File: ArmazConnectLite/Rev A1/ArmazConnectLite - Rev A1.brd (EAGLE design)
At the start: 56 x 24 mm, 17 parts, among them J1 22-05-7028-02, X1 MSTBA3, X8 87832-26

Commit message: Place copyright and board name
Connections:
- new net +24V: X1.1
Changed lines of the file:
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@@
 <contactref element="X8" pad="17"/>
+</signal>
+<signal name="+24V">
+<contactref element="X1" pad="1"/>
 </signal>
 </signals>

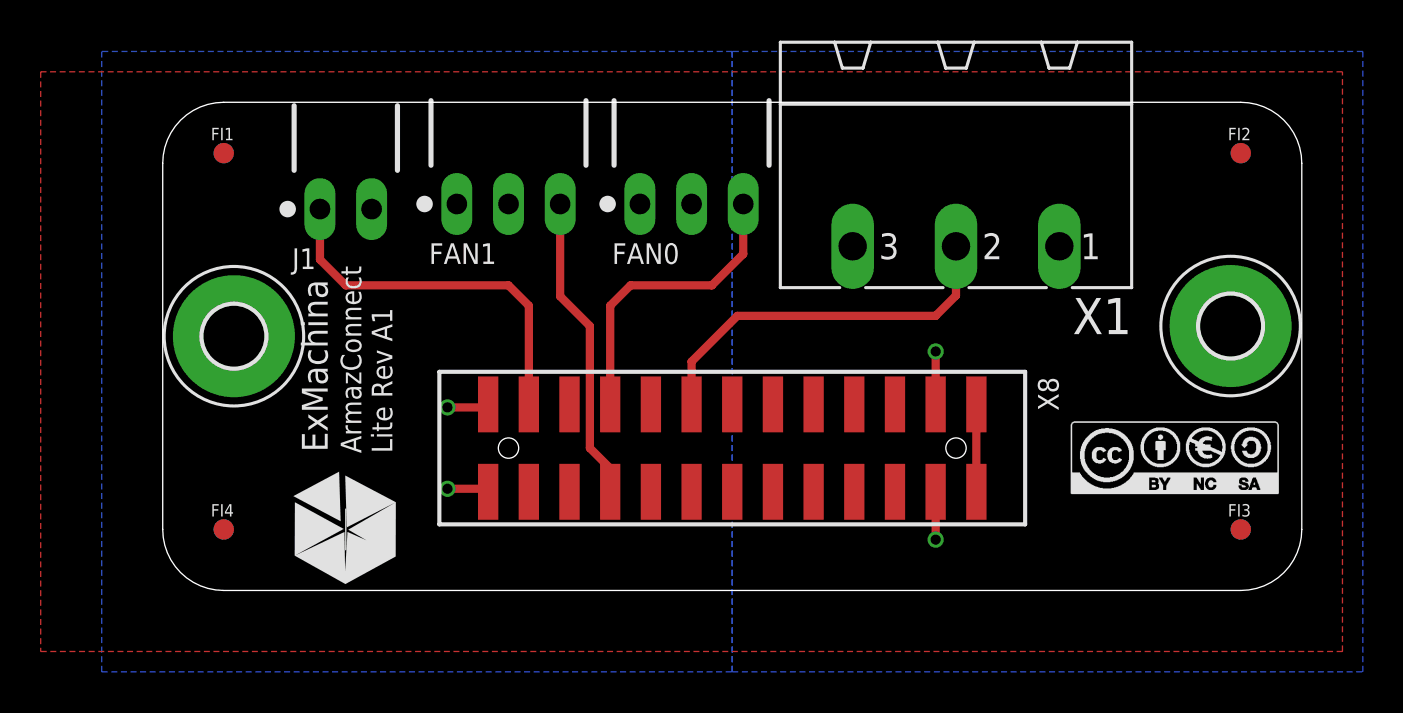
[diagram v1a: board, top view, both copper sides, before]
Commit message: generate gerber and MDP files
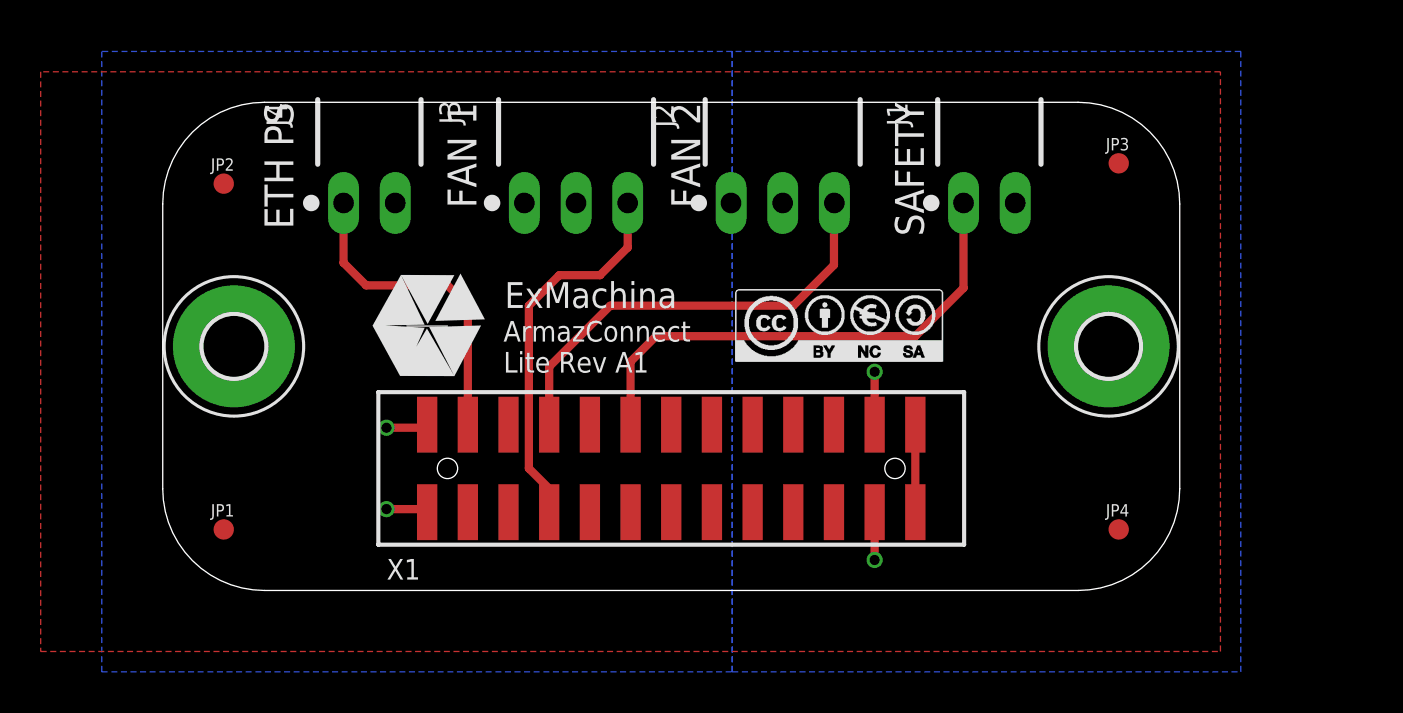
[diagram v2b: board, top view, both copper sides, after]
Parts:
- removed FAN0, FAN1: 22-05-7038-03, con-molex:7395-03
- removed FI1, FI2, FI3, FI4, FI5, FI6, FI7, FI8: FIDUCIAL1X2, SparkFun:FIDUCIAL-1X2
- removed U$1: EXMACHINA-LOGO-NAME, exmachina:EXM-LOGO-BASELINE
- removed X8: 87832-26, con-molex:87832-26
- added J2, J3: 22-05-7038-03, con-molex:7395-03
- added J4: 22-05-7028-02, con-molex:7395-02
- added JP1, JP2, JP3, JP4: FIDUCIAL1X2, SparkFun:FIDUCIAL-1X2
- added T1: EXMACHINA-LOGO-NAME, exmachina:EXM-LOGO-BASELINE
- added U$2: (no value), frames:A4L-LOC
- X1: value MSTBA3 -> 87832-26; device con-phoenix-508:MSTBA3 -> con-molex:87832-26
- moved MP1 49.0 mm to (3.50, 12.0)
- moved MP2 43.0 mm to (46.5, 12.0)
- moved J1 31.6 mm to (40.6, 19.1)
- moved X1 21.3 mm to (25.0, 6.00)
- moved CC1 17.7 mm to (33.2, 13.0)
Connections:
- removed net +24V: X1.1
- removed net VDD33A1: X8.24
- new net N$1: X1.24
- net +12V: now also J2.1, J3.1, X1.21, X1.22; no longer FAN0.1, FAN1.1, X8.21, X8.22
- net +5V: now also X1.1, X1.2; no longer X8.1, X8.2
- net +5V/1: now also J4.1, X1.23; no longer J1.1, X8.23
- net ESW0: now also X1.5; no longer X8.5
- net ESW1: now also X1.6; no longer X8.6
- net ESW2: now also X1.7; no longer X8.7
- net ESW3: now also X1.8; no longer X8.8
- net ESW4: now also J1.1, X1.15; no longer X1.2, X8.15
- net ESW5: now also X1.13; no longer X8.13
- net ESW6: now also X1.14; no longer X8.14
- net FAN0_GND: now also J2.3, X1.19; no longer FAN0.3, X8.19
- net FAN1_GND: now also J3.3, X1.20; no longer FAN1.3, X8.20
- net GND: now also J1.2, X1.4; no longer X8.3, X8.4
- net GND1: now also J4.2, X1.25, X1.26; no longer J1.2, X8.25, X8.26
- net OUT0: now also X1.16; no longer X8.16
- net OUT1: now also X1.17; no longer X8.17
- net OUT2: now also X1.18; no longer X8.18
- net UART4_RXD: now also X1.11; no longer X8.11
- net UART4_TXD: now also X1.12; no longer X8.12
- net UART5_RXD: now also X1.9; no longer X8.9
- net UART5_TXD: now also X1.10; no longer X8.10
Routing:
- net FAN0_GND: track 14.9 -> 22.0 mm
- net ESW4: track 18.9 -> 25.1 mm
- net FAN1_GND: track 15.2 -> 18.8 mm
- net +5V/1: track 18.5 -> 15.8 mm
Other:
- board size 56 x 24 mm -> 50 x 24 mm
- board text added: "ETH PS"
- board text added: "FAN 1"
- board text added: "FAN 2"
- board text added: "SAFETY"
- board text removed: "DMX0-IN"
- board text removed: "DMX0-OUT"
- board text removed: "DRV EN"
- board text removed: "ESW0"
- board text removed: "ESW1"
- board text removed: "ESW2"
- board text removed: "ESW3"
- board text removed: "ETH0-0"
